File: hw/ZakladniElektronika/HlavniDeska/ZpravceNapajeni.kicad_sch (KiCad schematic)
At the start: 7 parts, among them Q10 Q_PMOS_DGS, Q13 Q_PMOS_DGS

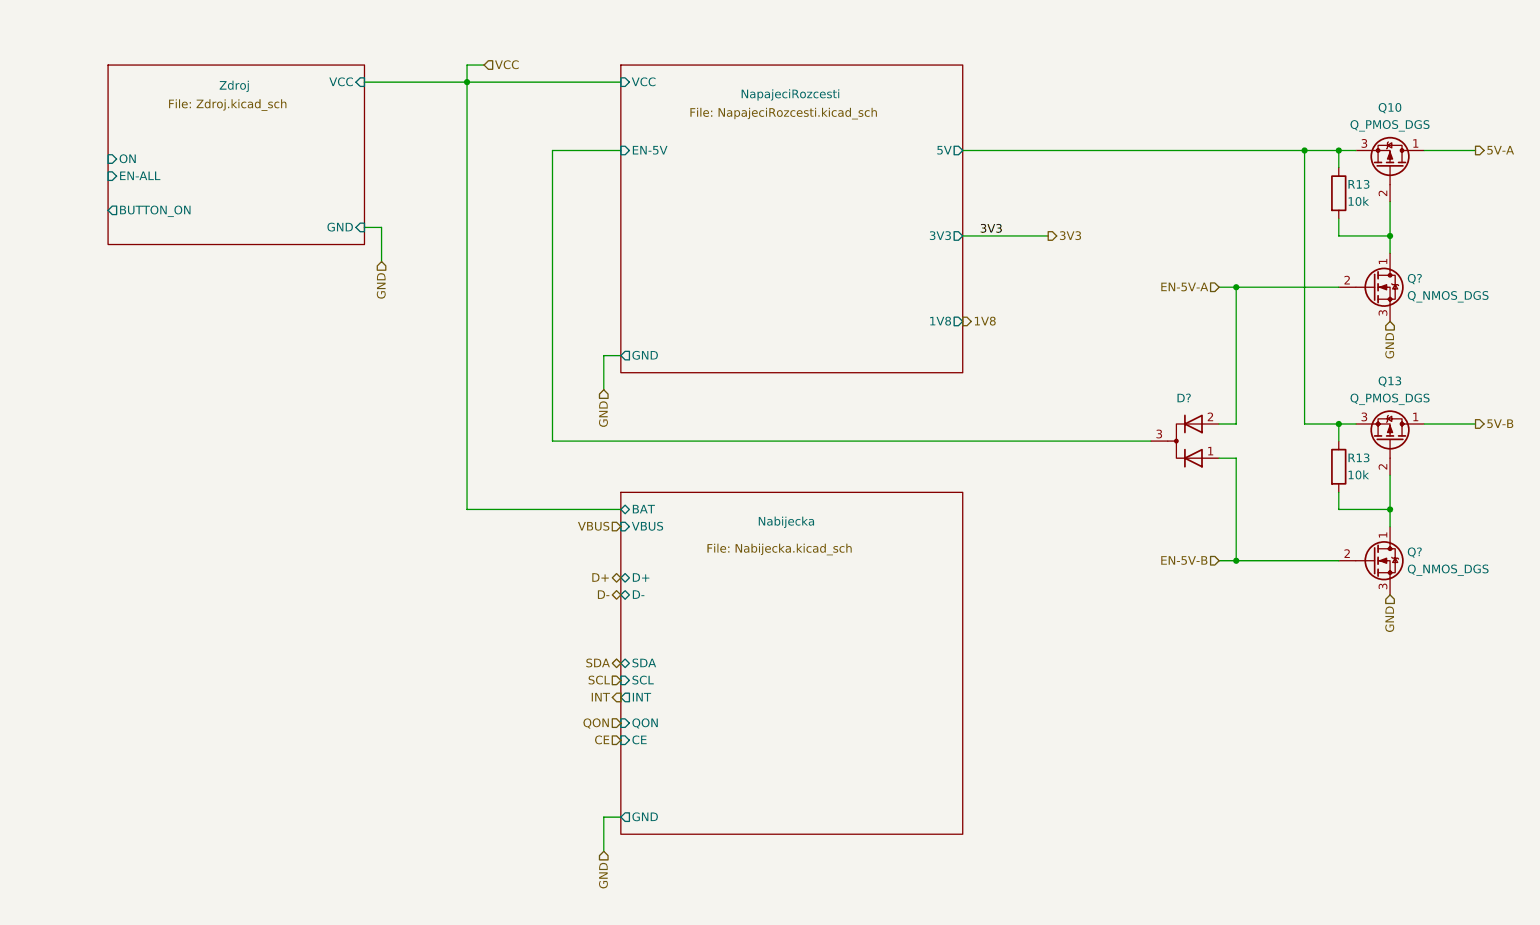
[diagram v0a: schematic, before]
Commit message: USB_multiplexer a přehlednost
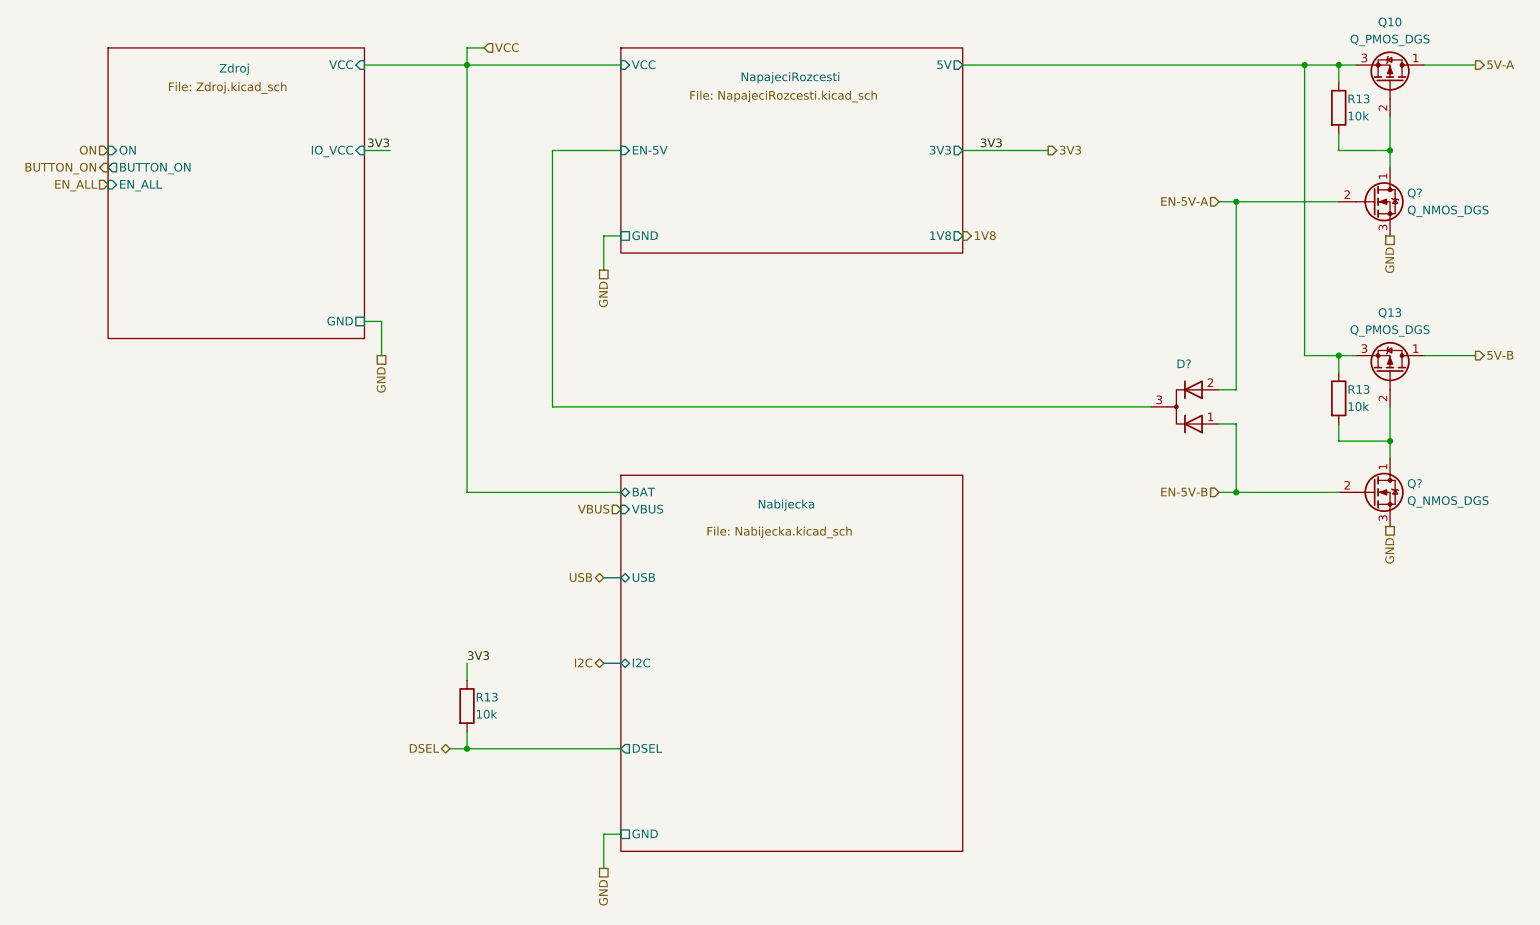
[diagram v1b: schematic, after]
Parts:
- added R13: 10k, Resistor_SMD:R_0402_1005Metric, symbol Device:R
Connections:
- net 3V3: now also R13.1
- new net DSEL: R13.2
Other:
- sheet Nabijecka ports: added DSEL, I2C, USB; removed CE, D+, D-, INT, QON, SCL, SDA
- sheet Zdroj ports: added EN_ALL, IO_VCC; removed EN-ALL
- moved on the sheet: D?, Q10, Q13, Q?, R13
